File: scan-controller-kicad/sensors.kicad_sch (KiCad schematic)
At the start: 23 parts, among them CN2 Shaft Eye, CN3 Film End Eye, J1 Shaft Eye, J2 Film End Eye, Q2 SS8050, U1 74LVC14, U2 QRE1113, U3 QRE1113

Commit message: 31 nets to go
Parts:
- TP7, TP8: footprint TestPoint:TestPoint_THTPad_D2.0mm_Drill1.0mm -> TestPoint:TestPoint_Pad_1.5x1.5mm
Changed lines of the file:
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@@
         )
         (path "/ab6dbce1-4ecf-44ae-8f33-5f07e4f43ca9/32afee9c-f78c-4810-b9e6-48288995c3da"
-          (reference "C15") (unit 1)
+          (reference "C14") (unit 1)
         )
       )
@@
         )
         (path "/ab6dbce1-4ecf-44ae-8f33-5f07e4f43ca9/32afee9c-f78c-4810-b9e6-48288995c3da"
-          (reference "C14") (unit 1)
+          (reference "C13") (unit 1)
         )
       )
@@
       (effects (font (size 1.27 1.27)) (justify left))
     )
-    (property "Footprint" "TestPoint:TestPoint_THTPad_D2.0mm_Drill1.0mm" (at 194.945 121.92 0)
+    (property "Footprint" "TestPoint:TestPoint_Pad_1.5x1.5mm" (at 194.945 121.92 0)
       (effects (font (size 1.27 1.27)) hide)
     )
@@
         )
         (path "/ab6dbce1-4ecf-44ae-8f33-5f07e4f43ca9/32afee9c-f78c-4810-b9e6-48288995c3da"
-          (reference "C13") (unit 1)
+          (reference "C12") (unit 1)
         )
       )
@@
       (effects (font (size 1.27 1.27)) (justify left))
     )
-    (property "Footprint" "TestPoint:TestPoint_THTPad_D2.0mm_Drill1.0mm" (at 194.31 76.2 0)
-      (effects (font (size 1.27 1.27)) hide)
-    )
+    (property "Footprint" "TestPoint:TestPoint_Pad_1.5x1.5mm" (at 194.31 76.2 0)
+      (effects (font (size 1.27 1.27)) hide)
+    )

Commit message: smaller eyes
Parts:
- R1, R5: footprint Resistor_SMD:R_0805_2012Metric -> Resistor_SMD:R_0402_1005Metric; LCSC C17408 -> C25076
- R10, R4: footprint Resistor_SMD:R_0805_2012Metric -> Resistor_SMD:R_0402_1005Metric; LCSC C17713 -> C25792
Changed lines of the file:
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@@
       (effects (font (size 1.27 1.27)) (justify left))
     )
-    (property "Footprint" "Resistor_SMD:R_0805_2012Metric" (at 107.315 69.215 0)
+    (property "Footprint" "Resistor_SMD:R_0402_1005Metric" (at 107.315 69.215 0)
       (effects (font (size 1.27 1.27)) hide)
     )
@@
       (effects (font (size 1.27 1.27)) hide)
     )
-    (property "LCSC" "C17713" (at 107.315 69.215 0)
+    (property "LCSC" "C25792" (at 107.315 69.215 0)
       (effects (font (size 1.27 1.27)) hide)
     )
@@
       (effects (font (size 1.27 1.27)) (justify left))
     )
-    (property "Footprint" "Resistor_SMD:R_0805_2012Metric" (at 92.71 114.935 0)
+    (property "Footprint" "Resistor_SMD:R_0402_1005Metric" (at 92.71 114.935 0)
       (effects (font (size 1.27 1.27)) hide)
     )
@@
       (effects (font (size 1.27 1.27)) hide)
     )
-    (property "LCSC" "C17408" (at 92.71 114.935 0)
+    (property "LCSC" "C25076" (at 92.71 114.935 0)
       (effects (font (size 1.27 1.27)) hide)
     )
@@
       (effects (font (size 1.27 1.27)) (justify left))
     )
-    (property "Footprint" "Resistor_SMD:R_0805_2012Metric" (at 107.95 114.935 0)
+    (property "Footprint" "Resistor_SMD:R_0402_1005Metric" (at 107.95 114.935 0)
       (effects (font (size 1.27 1.27)) hide)
     )
@@
       (effects (font (size 1.27 1.27)) hide)
     )
-    (property "LCSC" "C17713" (at 107.95 114.935 0)
+    (property "LCSC" "C25792" (at 107.95 114.935 0)
       (effects (font (size 1.27 1.27)) hide)
     )
@@
       (effects (font (size 1.27 1.27)) (justify left))
     )
-    (property "Footprint" "Resistor_SMD:R_0805_2012Metric" (at 92.075 69.215 0)
+    (property "Footprint" "Resistor_SMD:R_0402_1005Metric" (at 92.075 69.215 0)
       (effects (font (size 1.27 1.27)) hide)
     )
@@
       (effects (font (size 1.27 1.27)) hide)
     )
-    (property "LCSC" "C17408" (at 92.075 69.215 0)
-      (effects (font (size 1.27 1.27)) hide)
-    )
+    (property "LCSC" "C25076" (at 92.075 69.215 0)
+      (effects (font (size 1.27 1.27)) hide)
+    )

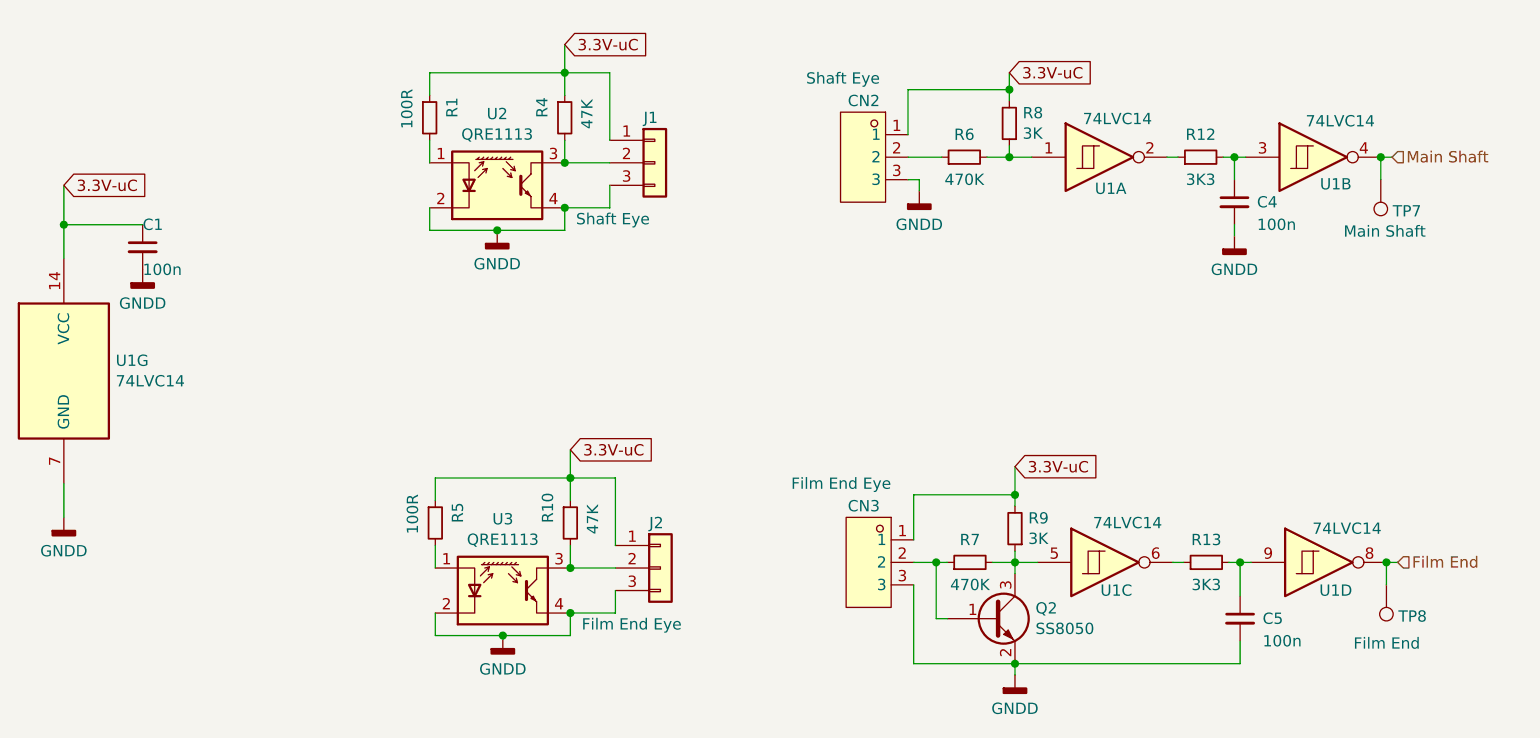
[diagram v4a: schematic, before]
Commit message: Round corners!
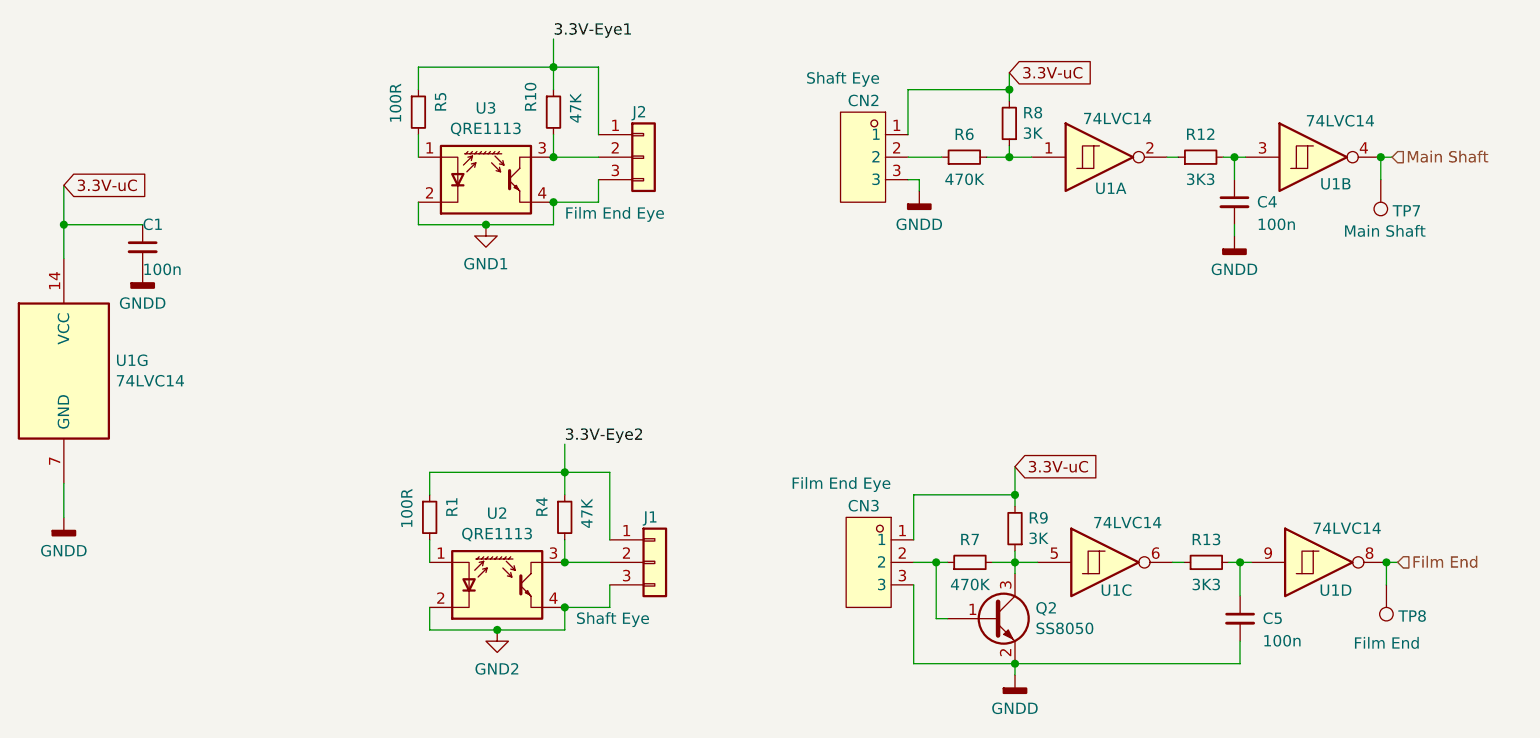
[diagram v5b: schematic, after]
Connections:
- net 3.3V-uC: no longer J1.1 (Pin_1), J2.1 (Pin_1), R1.1, R10.1, R4.1, R5.1
- net GNDD: no longer J1.3 (Pin_3), J2.3 (Pin_3), U2.2 (K), U2.4, U3.2 (K), U3.4
- new net 3.3V-Eye1: J2.1 (Pin_1), R10.1, R5.1
- new net 3.3V-Eye2: J1.1 (Pin_1), R1.1, R4.1
- new net GND1: J2.3 (Pin_3), U3.2 (K), U3.4
- new net GND2: J1.3 (Pin_3), U2.2 (K), U2.4
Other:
- moved on the sheet: J1, J2, R1, R10, R4, R5, U2, U3
